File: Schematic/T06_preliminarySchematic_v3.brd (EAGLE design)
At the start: 100 x 80 mm, 58 parts, among them Q3 2n3904, U1 ATMEGA328P_PDIP, X1 SSW-105-02-S-S, X2 SSW-102-02-S-S

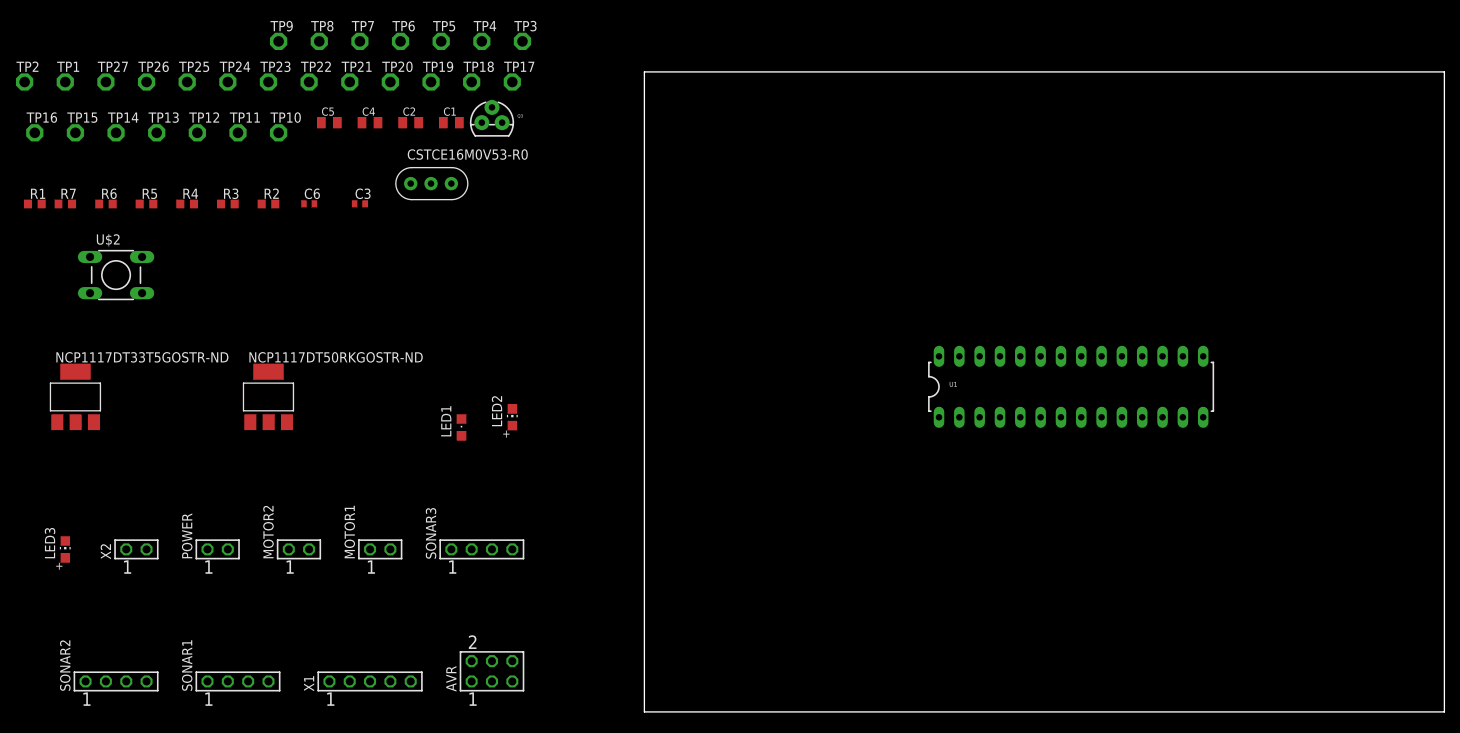
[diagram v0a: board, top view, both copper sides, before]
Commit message: still trying to figutr out git
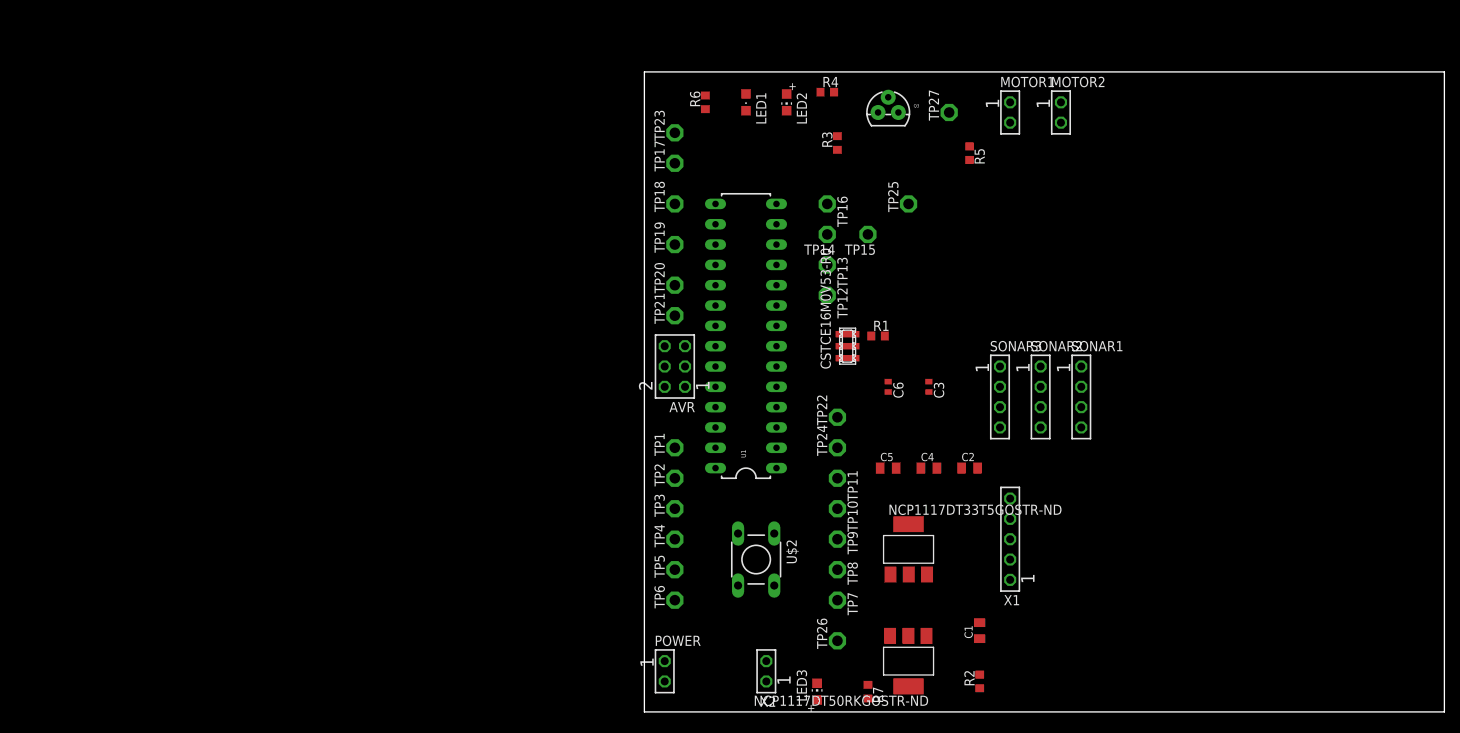
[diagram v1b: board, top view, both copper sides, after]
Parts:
- CSTCE16M0V53-R0: device adafruit:CERM_OSC -> adafruit:CSTCR-G
- moved SONAR2 120.9 mm to (49.5, 39.4), turned to 270 degrees
- moved R7 117.4 mm to (27.9, 2.54), turned to 270 degrees
- moved SONAR1 111.2 mm to (54.6, 39.4), turned to 270 degrees
- moved TP26 111.1 mm to (24.1, 8.89), turned to 90 degrees
- moved MOTOR2 109.8 mm to (52.1, 74.9), turned to 270 degrees
- moved R2 107.1 mm to (41.9, 3.81), turned to 90 degrees
- moved R1 106.7 mm to (29.2, 47.0)
- moved NCP1117DT33T5GOSTR-ND 105.9 mm to (33.0, 20.3)
- moved TP27 105.5 mm to (38.1, 74.9), turned to 90 degrees
- moved R5 103.1 mm to (40.6, 69.8), turned to 270 degrees
- moved TP15 99.9 mm to (27.9, 59.7), turned to 180 degrees
- moved TP16 99.5 mm to (22.9, 63.5), turned to 270 degrees
- moved MOTOR1 95.8 mm to (45.7, 74.9), turned to 270 degrees
- moved LED3 95.6 mm to (21.6, 2.54)
- moved TP2 95.2 mm to (3.81, 29.2), turned to 90 degrees
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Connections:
- net GND: now also CSTCE16M0V53-R0.2; no longer CSTCE16M0V53-R0.P$2
- net N$1: now also CSTCE16M0V53-R0.3; no longer CSTCE16M0V53-R0.P$3
- net N$2: now also CSTCE16M0V53-R0.1; no longer CSTCE16M0V53-R0.P$1

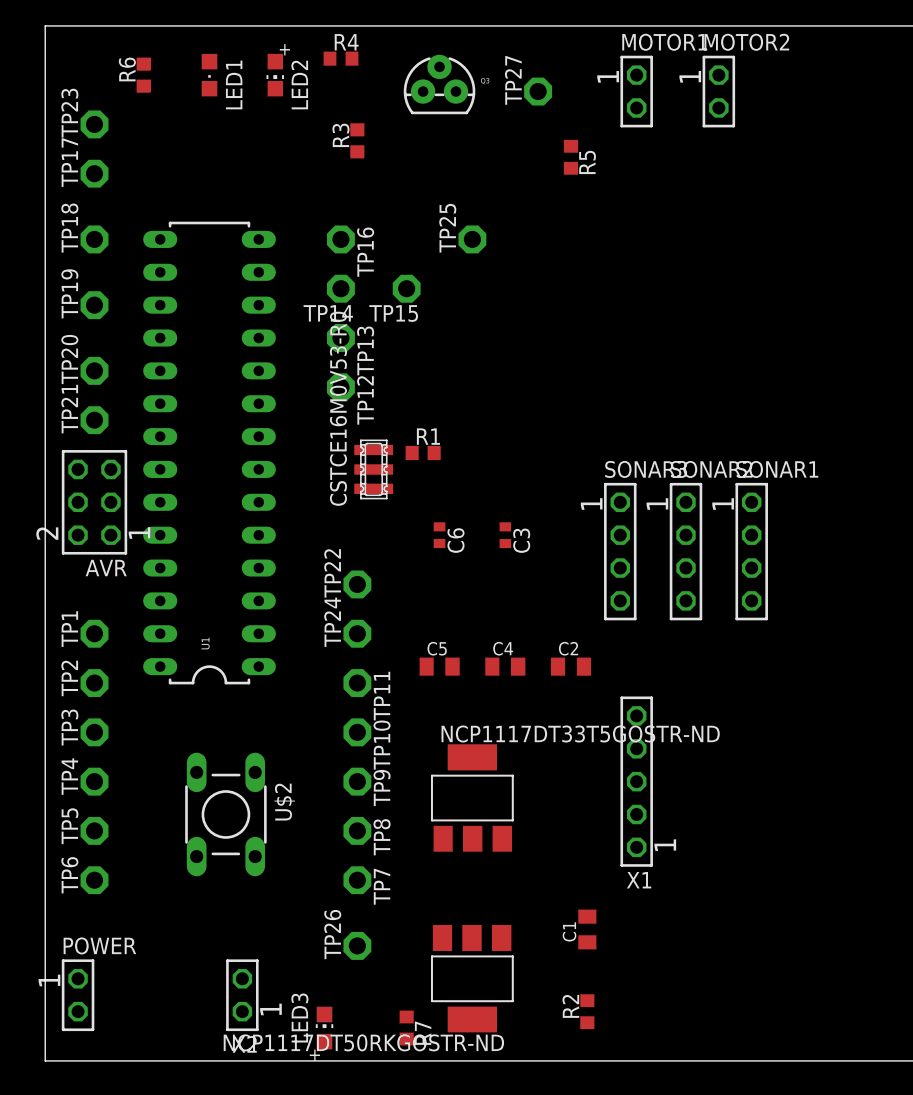
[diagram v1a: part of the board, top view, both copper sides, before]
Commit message: practice makes perfect
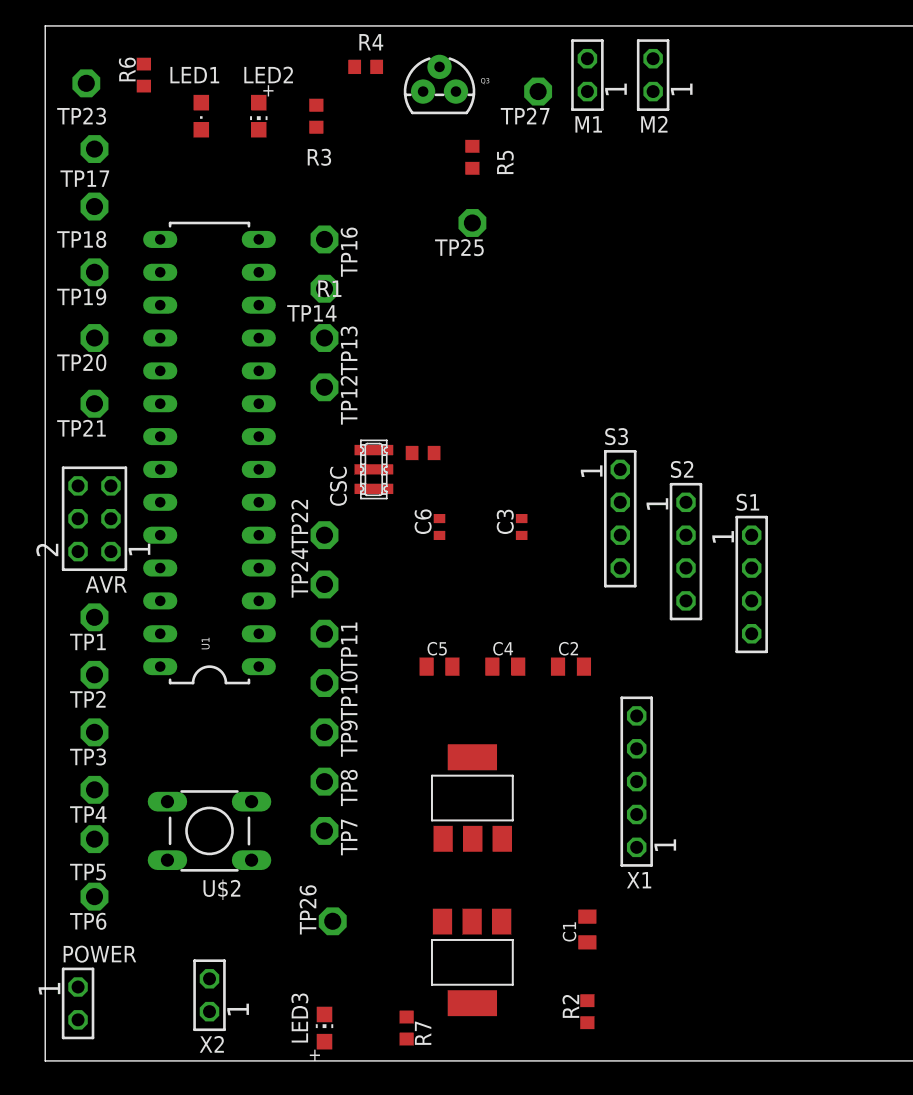
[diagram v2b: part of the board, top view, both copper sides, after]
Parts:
- removed MOTOR1, MOTOR2: SSW-102-02-S-S, con-samtec:SSW-102-02-S-S
- removed SONAR1, SONAR3: SSW-104-02-S-S, con-samtec:SSW-104-02-S-S
- removed TP15: TPPAD1-13, testpad:P1-13
- added M1, M2: SSW-102-02-S-S, con-samtec:SSW-102-02-S-S
- added S1, S3: SSW-104-02-S-S, con-samtec:SSW-104-02-S-S
- moved R5 7.62 mm to (33.0, 69.8)
- moved TP10 4.58 mm to (21.6, 29.2)
- moved TP11 4.58 mm to (21.6, 33.0)
- moved TP22 4.58 mm to (21.6, 40.6)
- moved TP7 4.58 mm to (21.6, 17.8)
- moved TP8 4.58 mm to (21.6, 21.6)
- moved TP9 4.58 mm to (21.6, 25.4)
- moved TP24 4.58 mm to (21.6, 36.8)
- moved R3 3.70 mm to (21.0, 73.0)
- moved LED2 3.42 mm to (16.5, 73.0)
- moved LED1 3.24 mm to (12.1, 73.0)
- moved TP23 3.24 mm to (3.17, 75.6), turned to 180 degrees
- moved TP26 2.69 mm to (22.2, 10.8)
- moved TP18 2.54 mm to (3.81, 66.0), turned to 180 degrees
- moved X2 2.54 mm to (12.7, 5.08)
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- renumbered CSTCE16M0V53-R0 to CSC, SONAR2 to S2
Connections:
- net +5V: now also S1.4, S3.4; no longer SONAR1.4, SONAR3.4
- net ECHO1: now also S1.2; no longer SONAR1.2
- net ECHO3: now also S3.2; no longer SONAR3.2, TP15.TP
- net GND: now also S1.1, S3.1; no longer SONAR1.1, SONAR3.1
- net N$11: now also M1.2, M2.2; no longer MOTOR1.2, MOTOR2.2
- net N$5: now also M1.1, M2.1; no longer MOTOR1.1, MOTOR2.1
- net TRIG: now also S1.3, S3.3; no longer SONAR1.3, SONAR3.3
